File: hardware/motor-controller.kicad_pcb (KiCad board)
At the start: 2 copper layers, 51 parts, among them P101 BATTERY, P102 SWD, P103 EDISON-BULB-E10, P104 FTDI-PLUG, P201 P06-MOTOR, P202 P06-MOTOR, U101 STM32F030K6T6, U102 ST-LIS3MDL, U201 IRLML2803TRPBF, U202 IRLML2803TRPBF, U203 7408, U204 MC33926, U205 MC33926, U206 74AHC541D

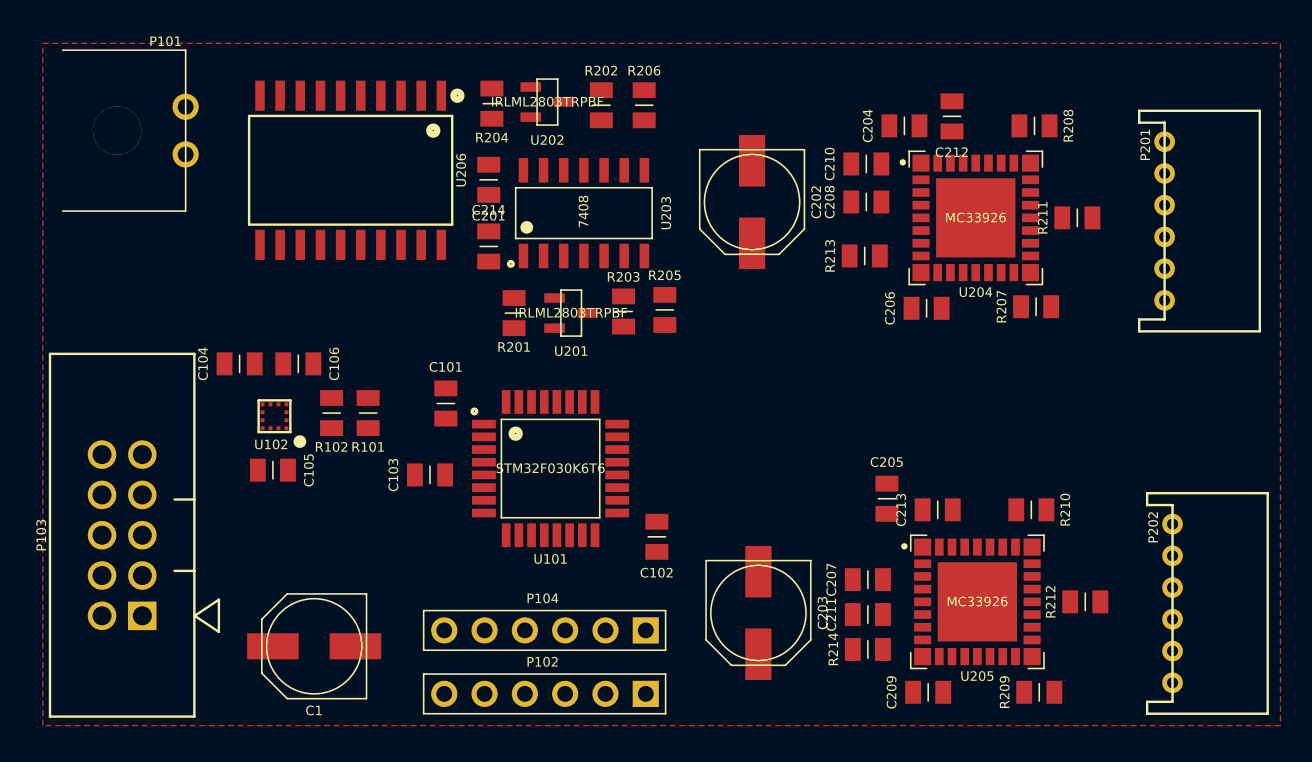
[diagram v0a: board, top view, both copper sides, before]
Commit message: initial layout
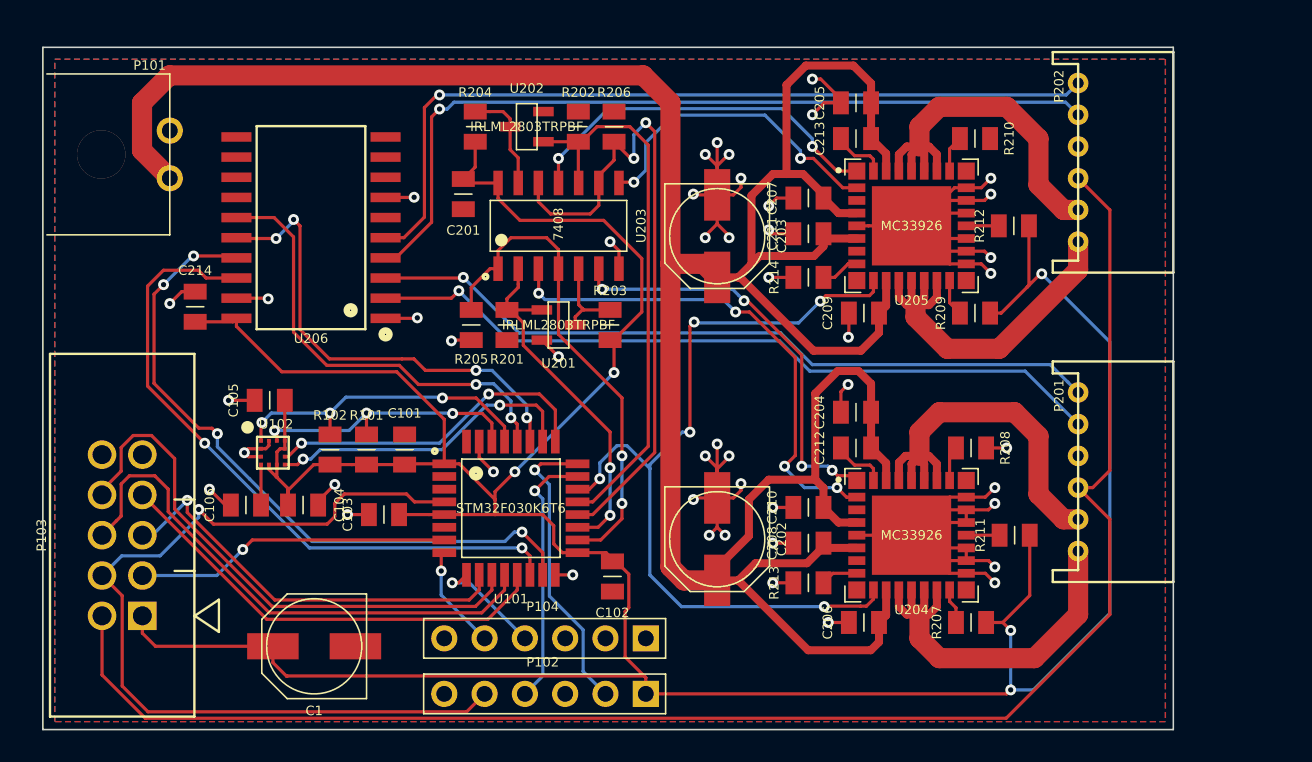
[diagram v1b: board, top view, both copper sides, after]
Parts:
- moved P202 28.4 mm to (178.2, 108.5)
- moved C205 25.0 mm to (164.2, 104.8), turned to 180 degrees
- moved C207 24.3 mm to (161.2, 110.8)
- moved C211 24.3 mm to (161.2, 113.0)
- moved C209 24.2 mm to (164.8, 118.0)
- moved R209 24.2 mm to (171.8, 118.0)
- moved R212 24.1 mm to (174.2, 112.5)
- moved U205 24.1 mm to (167.8, 112.5)
- moved C213 24.0 mm to (164.2, 107.0)
- moved C203 23.9 mm to (155.5, 113.2)
- moved R214 23.7 mm to (161.2, 115.8)
- moved R210 23.7 mm to (171.8, 107.0)
- moved C210 22.0 mm to (161.2, 130.2)
- moved C208 21.8 mm to (161.2, 132.5)
- moved C212 21.8 mm to (164.2, 126.5), turned to 180 degrees
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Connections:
- net Net-(P201-Pad1) renamed /drivers/MOTORL-
- net Net-(P201-Pad2) renamed /drivers/MOTORL+
- net Net-(P202-Pad1) renamed /drivers/MOTORR-
- net Net-(P202-Pad2) renamed /drivers/MOTORR+
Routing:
- net +3.3V: track 0.00 -> 216.6 mm, vias 0 -> 5
- net Vcc: track 0.00 -> 187.9 mm
- net GNDPWR: track 0.00 -> 149.5 mm, vias 0 -> 48
- net +5V: track 0.00 -> 101.6 mm
- net /NRST: track 0.00 -> 56.9 mm, vias 0 -> 1
- net /drivers/MOTOREN: track 0.00 -> 52.8 mm, vias 0 -> 5
- net Net-(P202-Pad5): track 0.00 -> 51.9 mm, vias 0 -> 1
- net Net-(P202-Pad6): track 0.00 -> 51.7 mm, vias 0 -> 1
- net Net-(P201-Pad5): track 0.00 -> 47.3 mm, vias 0 -> 1
- net Net-(P201-Pad6): track 0.00 -> 46.7 mm, vias 0 -> 1
- net /drivers/MOTORLCHB: track 0.00 -> 43.2 mm, vias 0 -> 4
- net /drivers/MOTORLCHA: track 0.00 -> 42.2 mm, vias 0 -> 2
- net /drivers/MOTORRPWM: track 0.00 -> 41.7 mm, vias 0 -> 2
- net /drivers/MOTORRDIR: track 0.00 -> 35.0 mm
- net /SPISCK: track 0.00 -> 34.9 mm
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- added copper zone on B.Cu, net GNDPWR
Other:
- board outline added: 71.2 x 43 mm
- net class Default: clearance 0.2 -> 0.2032; trace_width 0.25 -> 0.2032; via_dia 0.6 -> 0.6858; via_drill 0.4 -> 0.3302
- net class VCC added: clearance 0.254, trace_width 0.508, via_dia 0.6858, via_drill 0.3302
- rule trace_clearance: 0.2 -> 0.2032
